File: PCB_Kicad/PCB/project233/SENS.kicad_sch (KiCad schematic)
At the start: 6 parts, among them U2 MAX30102EFD_

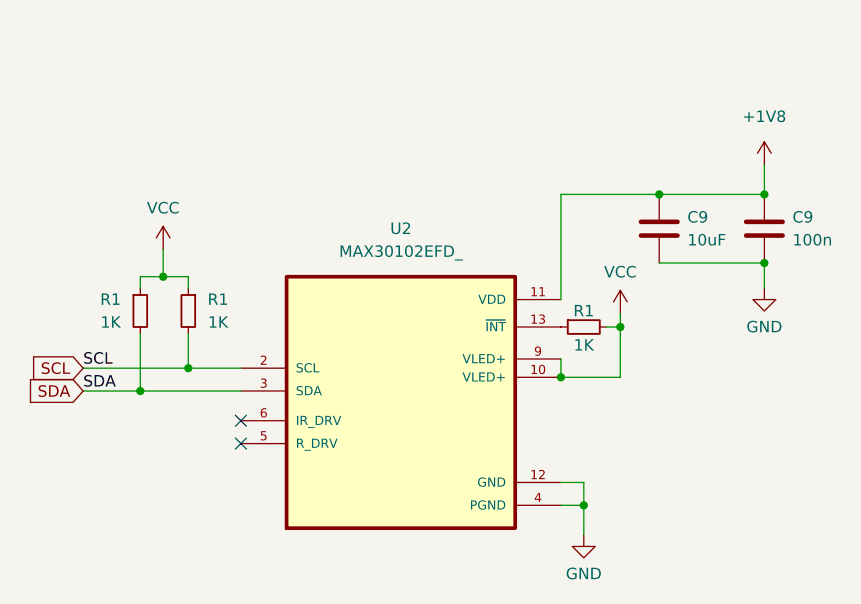
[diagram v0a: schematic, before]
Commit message: update KICAD PCB
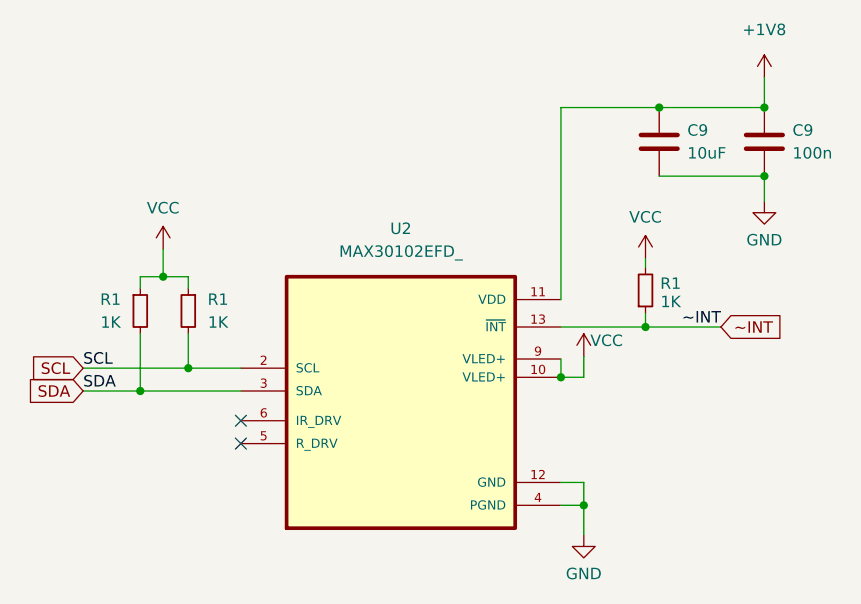
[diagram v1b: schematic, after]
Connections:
- net ~INT: now reaches R1.1, U2.13 (~{INT})
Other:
- moved on the sheet: C9, R1
